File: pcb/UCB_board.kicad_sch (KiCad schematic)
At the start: 29 parts

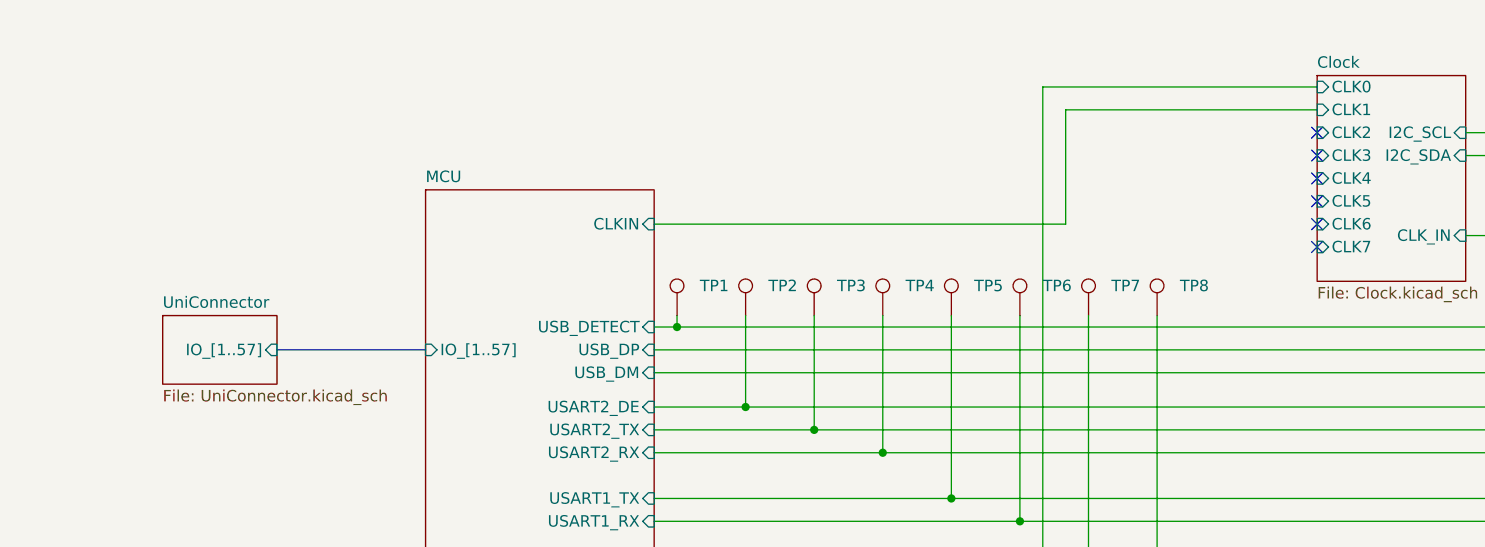
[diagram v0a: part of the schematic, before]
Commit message: Clock rounting
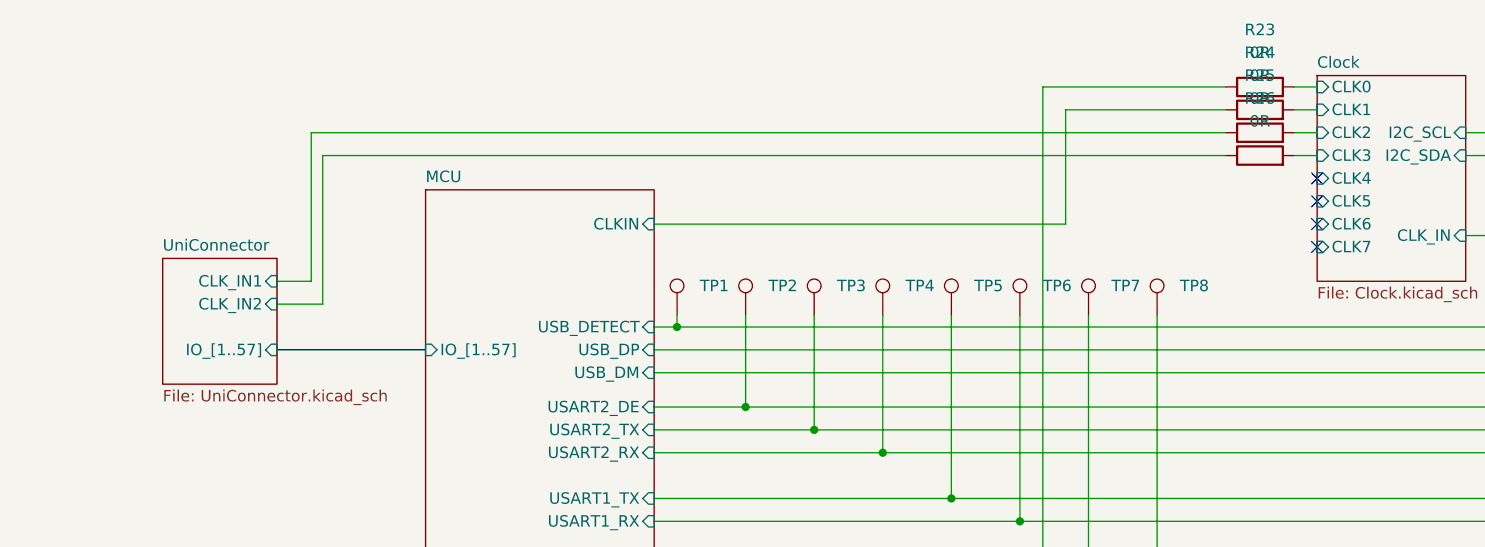
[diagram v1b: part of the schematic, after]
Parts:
- added R23, R24, R25, R26: 0R, Resistor_SMD:R_0402_1005Metric_Pad0.72x0.64mm_HandSolder, symbol Device:R
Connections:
- net Clock/CLK0: now also R23.2; no longer TP12.1
- net Clock/CLK1: now also R24.2
- net Clock/CLK2: now also R25.2
- net Clock/CLK3: now also R26.2
- new net EthernetPHY/CLKIN: R23.1, TP12.1
- new net MCU/CLKIN: R24.1
- new net UniConnector/CLK_IN1: R25.1
- new net UniConnector/CLK_IN2: R26.1
- no-connect marks 6 -> 4
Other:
- sheet UniConnector ports: added CLK_IN1, CLK_IN2; removed none
